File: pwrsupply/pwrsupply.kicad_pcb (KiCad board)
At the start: 2 copper layers, 33 x 24.1 mm, 9 parts, among them J1 Conn_01x02, J2 Conn_01x04, U1 LM2904, U2 L7809, U3 LM7909_TO220

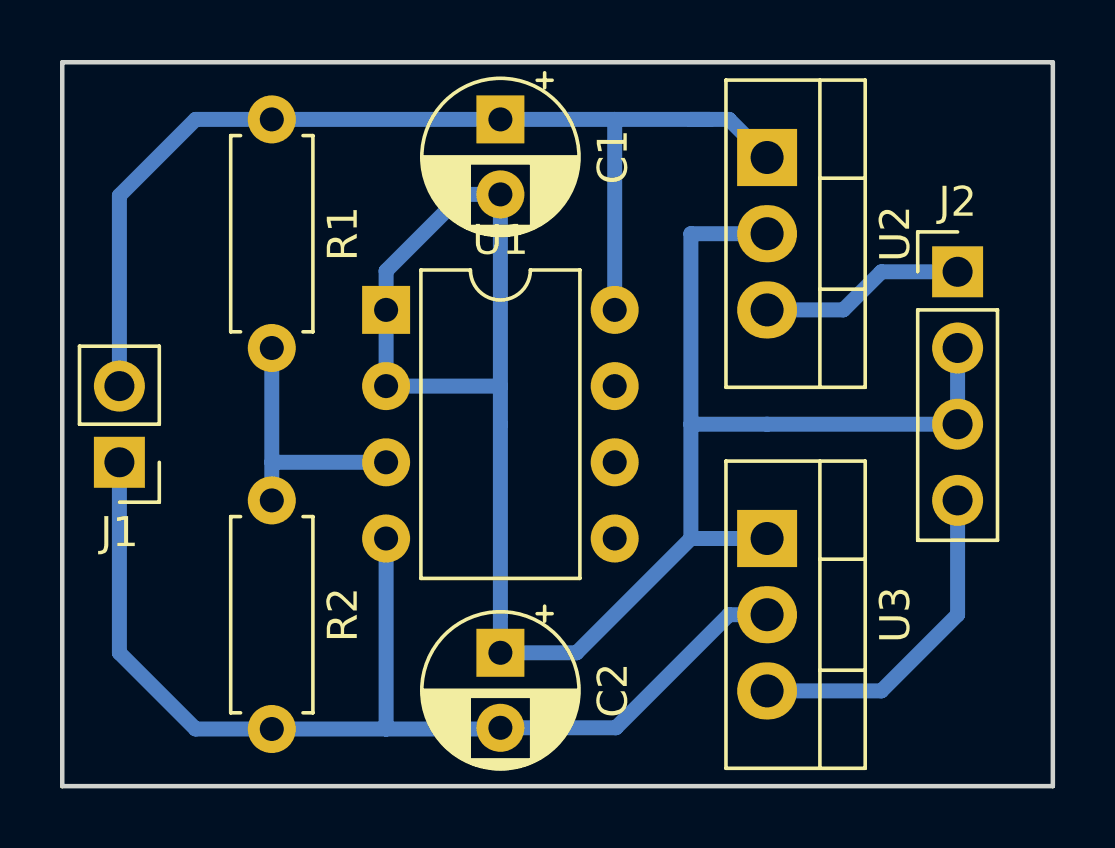
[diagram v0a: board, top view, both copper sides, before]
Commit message: updates
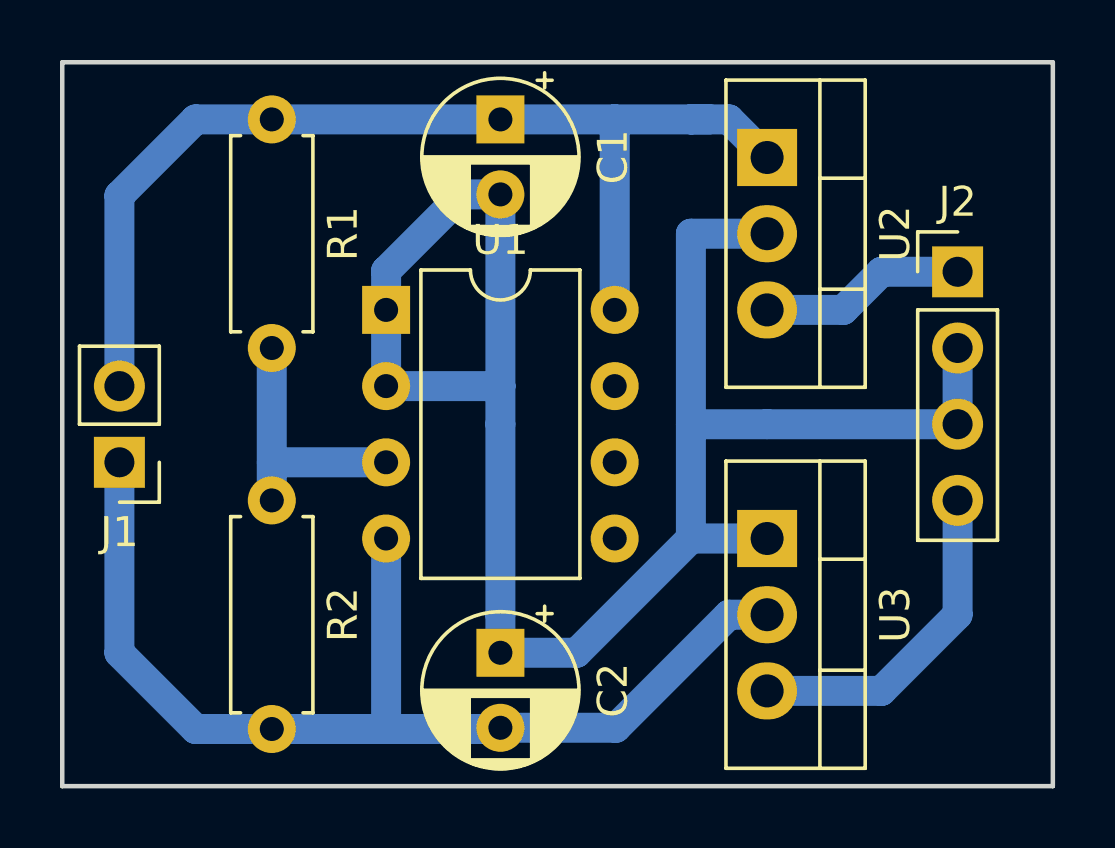
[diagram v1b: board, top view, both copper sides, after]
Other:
- net class Default: clearance 0.2 -> 0.3; trace_width 0.5 -> 1
- rule trace_clearance: 0.2 -> 0.3
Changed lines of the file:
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@@
   )
   (setup
-    (last_trace_width 0.5)
-    (trace_clearance 0.2)
+    (last_trace_width 1)
+    (trace_clearance 0.3)
     (zone_clearance 0.508)
     (zone_45_only no)
@@
   (net 6 "Net-(J2-Pad4)")
   (net_class Default "This is the default net class."
-    (clearance 0.2)
-    (trace_width 0.5)
+    (clearance 0.3)
+    (trace_width 1)
     (via_dia 0.8)
     (via_drill 0.4)
@@
   (gr_line (start 88.265 86.995) (end 88.265 62.865) (layer Margin) (width 0.2))
   (target plus (at 88.265 86.995) (size 5) (width 0.15) (layer Edge.Cuts))
-  (segment (start 90.17 73.66) (end 90.17 67.31) (width 0.5) (layer B.Cu) (net 1))
-  (segment (start 90.17 67.31) (end 92.71 64.77) (width 0.5) (layer B.Cu) (net 1))
-  (segment (start 92.71 64.77) (end 95.25 64.77) (width 0.5) (layer B.Cu) (net 1))
-  (segment (start 95.25 64.77) (end 102.87 64.77) (width 0.5) (layer B.Cu) (net 1))
-  (segment (start 106.68 71.12) (end 106.68 64.77) (width 0.5) (layer B.Cu) (net 1))
-  (segment (start 102.87 64.77) (end 106.68 64.77) (width 0.5) (layer B.Cu) (net 1))
-  (segment (start 111.76 66.04) (end 110.49 64.77) (width 0.5) (layer B.Cu) (net 1))
-  (segment (start 110.49 64.77) (end 109.22 64.77) (width 0.5) (layer B.Cu) (net 1))
-  (segment (start 106.68 64.77) (end 109.22 64.77) (width 0.5) (layer B.Cu) (net 1))
-  (segment (start 109.22 64.77) (end 109.855 64.77) (width 0.5) (layer B.Cu) (net 1))
-  (segment (start 99.06 73.66) (end 99.06 71.12) (width 0.5) (layer B.Cu) (net 2))
-  (segment (start 101.61 67.27) (end 102.87 67.27) (width 0.5) (layer B.Cu) (net 2))
-  (segment (start 99.06 71.12) (end 99.06 69.82) (width 0.5) (layer B.Cu) (net 2))
-  (segment (start 99.06 69.82) (end 101.61 67.27) (width 0.5) (layer B.Cu) (net 2))
-  (segment (start 99.06 73.66) (end 102.87 73.66) (width 0.5) (layer B.Cu) (net 2))
-  (segment (start 102.87 67.27) (end 102.87 73.66) (width 0.5) (layer B.Cu) (net 2))
-  (segment (start 118.11 74.93) (end 111.76 74.93) (width 0.5) (layer B.Cu) (net 2))
-  (segment (start 111.76 74.93) (end 109.22 74.93) (width 0.5) (layer B.Cu) (net 2))
-  (segment (start 102.87 74.93) (end 102.87 73.66) (width 0.5) (layer B.Cu) (net 2))
-  (segment (start 102.87 81.28) (end 102.87 74.93) (width 0.5) (layer B.Cu) (net 2))
-  (segment (start 102.87 82.55) (end 102.87 81.28) (width 0.5) (layer B.Cu) (net 2))
-  (segment (start 111.76 78.74) (end 109.22 78.74) (width 0.5) (layer B.Cu) (net 2))
-  (segment (start 109.22 74.93) (end 109.22 78.74) (width 0.5) (layer B.Cu) (net 2))
-  (segment (start 102.87 82.55) (end 105.41 82.55) (width 0.5) (layer B.Cu) (net 2))
-  (segment (start 105.41 82.55) (end 109.22 78.74) (width 0.5) (layer B.Cu) (net 2))
-  (segment (start 118.11 74.93) (end 118.11 72.39) (width 0.5) (layer B.Cu) (net 2))
-  (segment (start 109.22 68.58) (end 109.22 74.93) (width 0.5) (layer B.Cu) (net 2))
-  (segment (start 111.76 68.58) (end 109.22 68.58) (width 0.5) (layer B.Cu) (net 2))
-  (segment (start 102.83 85.09) (end 102.87 85.05) (width 0.5) (layer B.Cu) (net 3))
-  (segment (start 90.17 76.2) (end 90.17 82.55) (width 0.5) (layer B.Cu) (net 3))
-  (segment (start 92.71 85.09) (end 95.25 85.09) (width 0.5) (layer B.Cu) (net 3))
-  (segment (start 90.17 82.55) (end 92.71 85.09) (width 0.5) (layer B.Cu) (net 3))
-  (segment (start 99.06 78.74) (end 99.06 85.09) (width 0.5) (layer B.Cu) (net 3))
-  (segment (start 95.25 85.09) (end 99.06 85.09) (width 0.5) (layer B.Cu) (net 3))
-  (segment (start 99.06 85.09) (end 102.83 85.09) (width 0.5) (layer B.Cu) (net 3))
-  (segment (start 102.87 85.05) (end 106.72 85.05) (width 0.5) (layer B.Cu) (net 3))
-  (segment (start 106.72 85.05) (end 110.49 81.28) (width 0.5) (layer B.Cu) (net 3))
-  (segment (start 110.49 81.28) (end 111.76 81.28) (width 0.5) (layer B.Cu) (net 3))
-  (segment (start 111.76 71.12) (end 114.3 71.12) (width 0.5) (layer B.Cu) (net 4))
-  (segment (start 115.57 69.85) (end 118.11 69.85) (width 0.5) (layer B.Cu) (net 4))
-  (segment (start 114.3 71.12) (end 115.57 69.85) (width 0.5) (layer B.Cu) (net 4))
-  (segment (start 95.25 72.39) (end 95.25 77.47) (width 0.5) (layer B.Cu) (net 5))
-  (segment (start 99.06 76.2) (end 95.25 76.2) (width 0.5) (layer B.Cu) (net 5))
-  (segment (start 118.11 81.28) (end 118.11 77.47) (width 0.5) (layer B.Cu) (net 6))
-  (segment (start 111.76 83.82) (end 115.57 83.82) (width 0.5) (layer B.Cu) (net 6))
-  (segment (start 115.57 83.82) (end 118.11 81.28) (width 0.5) (layer B.Cu) (net 6))
+  (segment (start 90.17 73.66) (end 90.17 67.31) (width 1) (layer B.Cu) (net 1))
+  (segment (start 92.71 64.77) (end 95.25 64.77) (width 1) (layer B.Cu) (net 1))
+  (segment (start 90.17 67.31) (end 92.71 64.77) (width 1) (layer B.Cu) (net 1))
+  (segment (start 95.25 64.77) (end 102.87 64.77) (width 1) (layer B.Cu) (net 1))
+  (segment (start 106.68 71.12) (end 106.68 64.77) (width 1) (layer B.Cu) (net 1))
+  (segment (start 102.87 64.77) (end 106.68 64.77) (width 1) (layer B.Cu) (net 1))
+  (segment (start 111.76 66.04) (end 110.49 64.77) (width 1) (layer B.Cu) (net 1))
+  (segment (start 110.49 64.77) (end 109.22 64.77) (width 1) (layer B.Cu) (net 1))
+  (segment (start 106.68 64.77) (end 109.22 64.77) (width 1) (layer B.Cu) (net 1))
+  (segment (start 109.22 64.77) (end 109.855 64.77) (width 1) (layer B.Cu) (net 1))
+  (segment (start 99.06 73.66) (end 99.06 71.12) (width 1) (layer B.Cu) (net 2))
+  (segment (start 101.61 67.27) (end 102.87 67.27) (width 1) (layer B.Cu) (net 2))
+  (segment (start 99.06 71.12) (end 99.06 69.82) (width 1) (layer B.Cu) (net 2))
+  (segment (start 99.06 69.82) (end 101.61 67.27) (width 1) (layer B.Cu) (net 2))
+  (segment (start 99.06 73.66) (end 102.87 73.66) (width 1) (layer B.Cu) (net 2))
+  (segment (start 102.87 67.27) (end 102.87 73.66) (width 1) (layer B.Cu) (net 2))
+  (segment (start 118.11 74.93) (end 111.76 74.93) (width 1) (layer B.Cu) (net 2))
+  (segment (start 111.76 74.93) (end 109.22 74.93) (width 1) (layer B.Cu) (net 2))
+  (segment (start 102.87 74.93) (end 102.87 73.66) (width 1) (layer B.Cu) (net 2))
+  (segment (start 102.87 81.28) (end 102.87 74.93) (width 1) (layer B.Cu) (net 2))
+  (segment (start 102.87 82.55) (end 102.87 81.28) (width 1) (layer B.Cu) (net 2))
+  (segment (start 111.76 78.74) (end 109.22 78.74) (width 1) (layer B.Cu) (net 2))
+  (segment (start 109.22 74.93) (end 109.22 78.74) (width 1) (layer B.Cu) (net 2))
+  (segment (start 102.87 82.55) (end 105.41 82.55) (width 1) (layer B.Cu) (net 2))
+  (segment (start 105.41 82.55) (end 109.22 78.74) (width 1) (layer B.Cu) (net 2))
+  (segment (start 118.11 74.93) (end 118.11 72.39) (width 1) (layer B.Cu) (net 2))
+  (segment (start 109.22 68.58) (end 109.22 74.93) (width 1) (layer B.Cu) (net 2))
+  (segment (start 111.76 68.58) (end 109.22 68.58) (width 1) (layer B.Cu) (net 2))
+  (segment (start 102.83 85.09) (end 102.87 85.05) (width 1) (layer B.Cu) (net 3))
+  (segment (start 90.17 76.2) (end 90.17 82.55) (width 1) (layer B.Cu) (net 3))
+  (segment (start 92.71 85.09) (end 95.25 85.09) (width 1) (layer B.Cu) (net 3))
+  (segment (start 90.17 82.55) (end 92.71 85.09) (width 1) (layer B.Cu) (net 3))
+  (segment (start 99.06 78.74) (end 99.06 85.09) (width 1) (layer B.Cu) (net 3))
+  (segment (start 95.25 85.09) (end 99.06 85.09) (width 1) (layer B.Cu) (net 3))
+  (segment (start 99.06 85.09) (end 102.83 85.09) (width 1) (layer B.Cu) (net 3))
+  (segment (start 102.87 85.05) (end 106.72 85.05) (width 1) (layer B.Cu) (net 3))
+  (segment (start 106.72 85.05) (end 110.49 81.28) (width 1) (layer B.Cu) (net 3))
+  (segment (start 110.49 81.28) (end 111.76 81.28) (width 1) (layer B.Cu) (net 3))
+  (segment (start 111.76 71.12) (end 114.3 71.12) (width 1) (layer B.Cu) (net 4))
+  (segment (start 115.57 69.85) (end 118.11 69.85) (width 1) (layer B.Cu) (net 4))
+  (segment (start 114.3 71.12) (end 115.57 69.85) (width 1) (layer B.Cu) (net 4))
+  (segment (start 95.25 72.39) (end 95.25 77.47) (width 1) (layer B.Cu) (net 5))
+  (segment (start 99.06 76.2) (end 95.25 76.2) (width 1) (layer B.Cu) (net 5))
+  (segment (start 118.11 81.28) (end 118.11 77.47) (width 1) (layer B.Cu) (net 6))
+  (segment (start 111.76 83.82) (end 115.57 83.82) (width 1) (layer B.Cu) (net 6))
+  (segment (start 115.57 83.82) (end 118.11 81.28) (width 1) (layer B.Cu) (net 6))
 )
